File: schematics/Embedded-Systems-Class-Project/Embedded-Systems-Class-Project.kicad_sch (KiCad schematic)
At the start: 20 parts

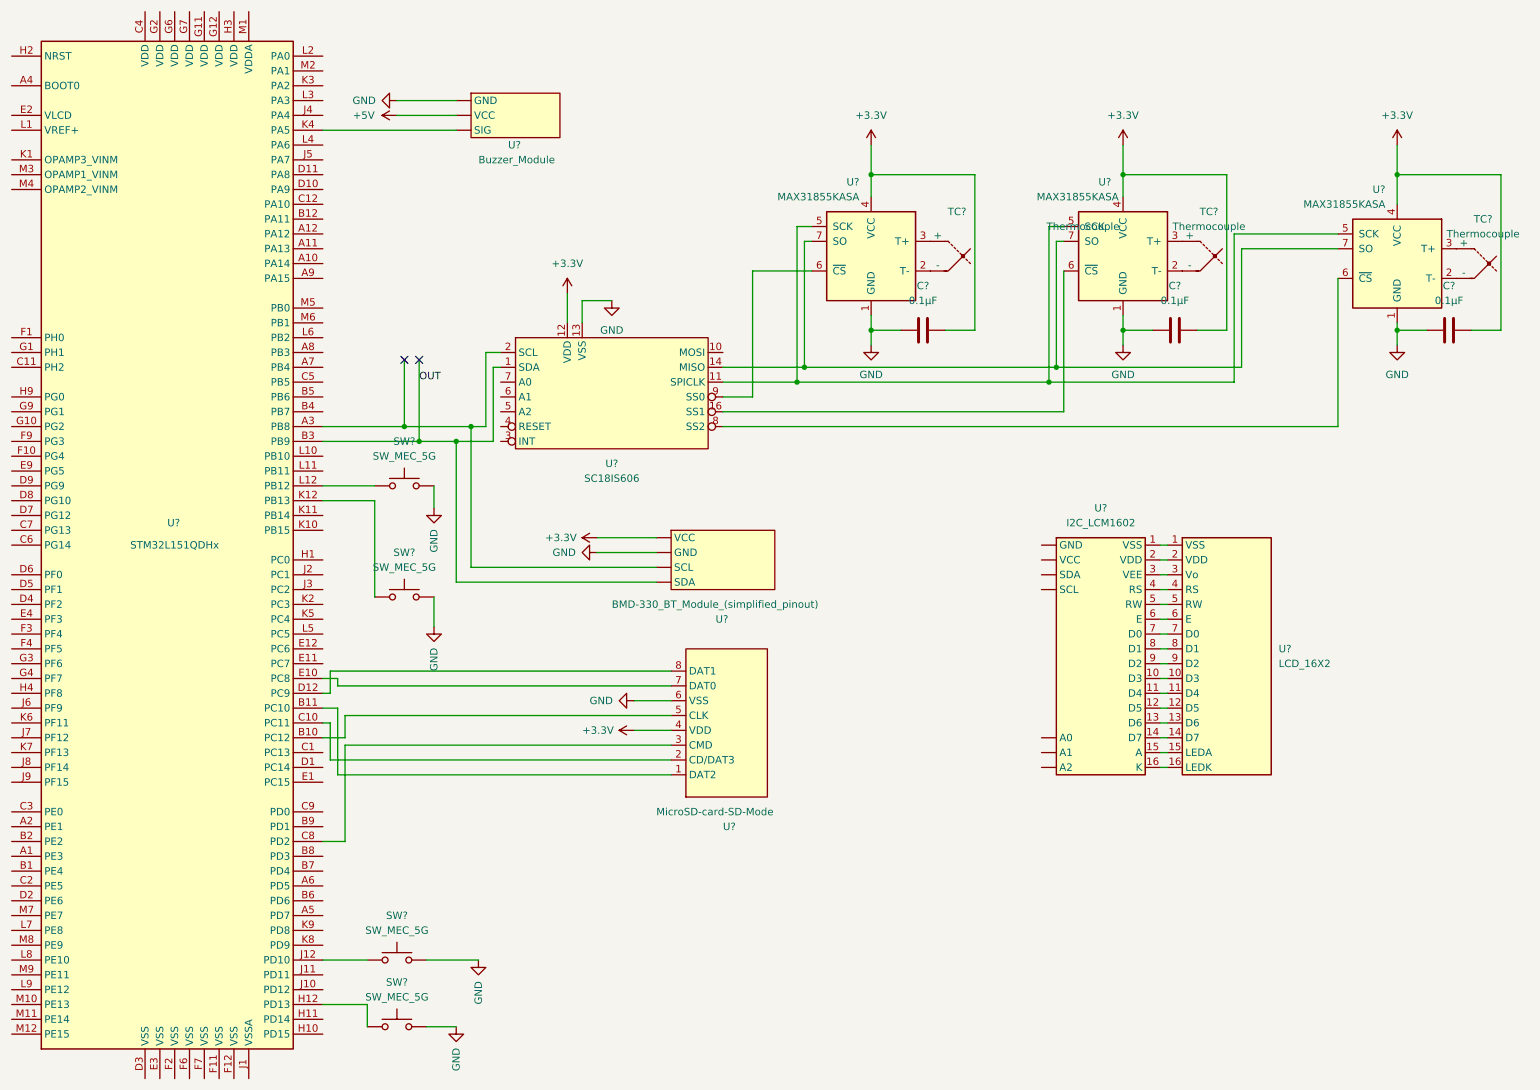
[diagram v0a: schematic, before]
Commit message: Update Embedded-Systems-Class-Project.kicad_sch
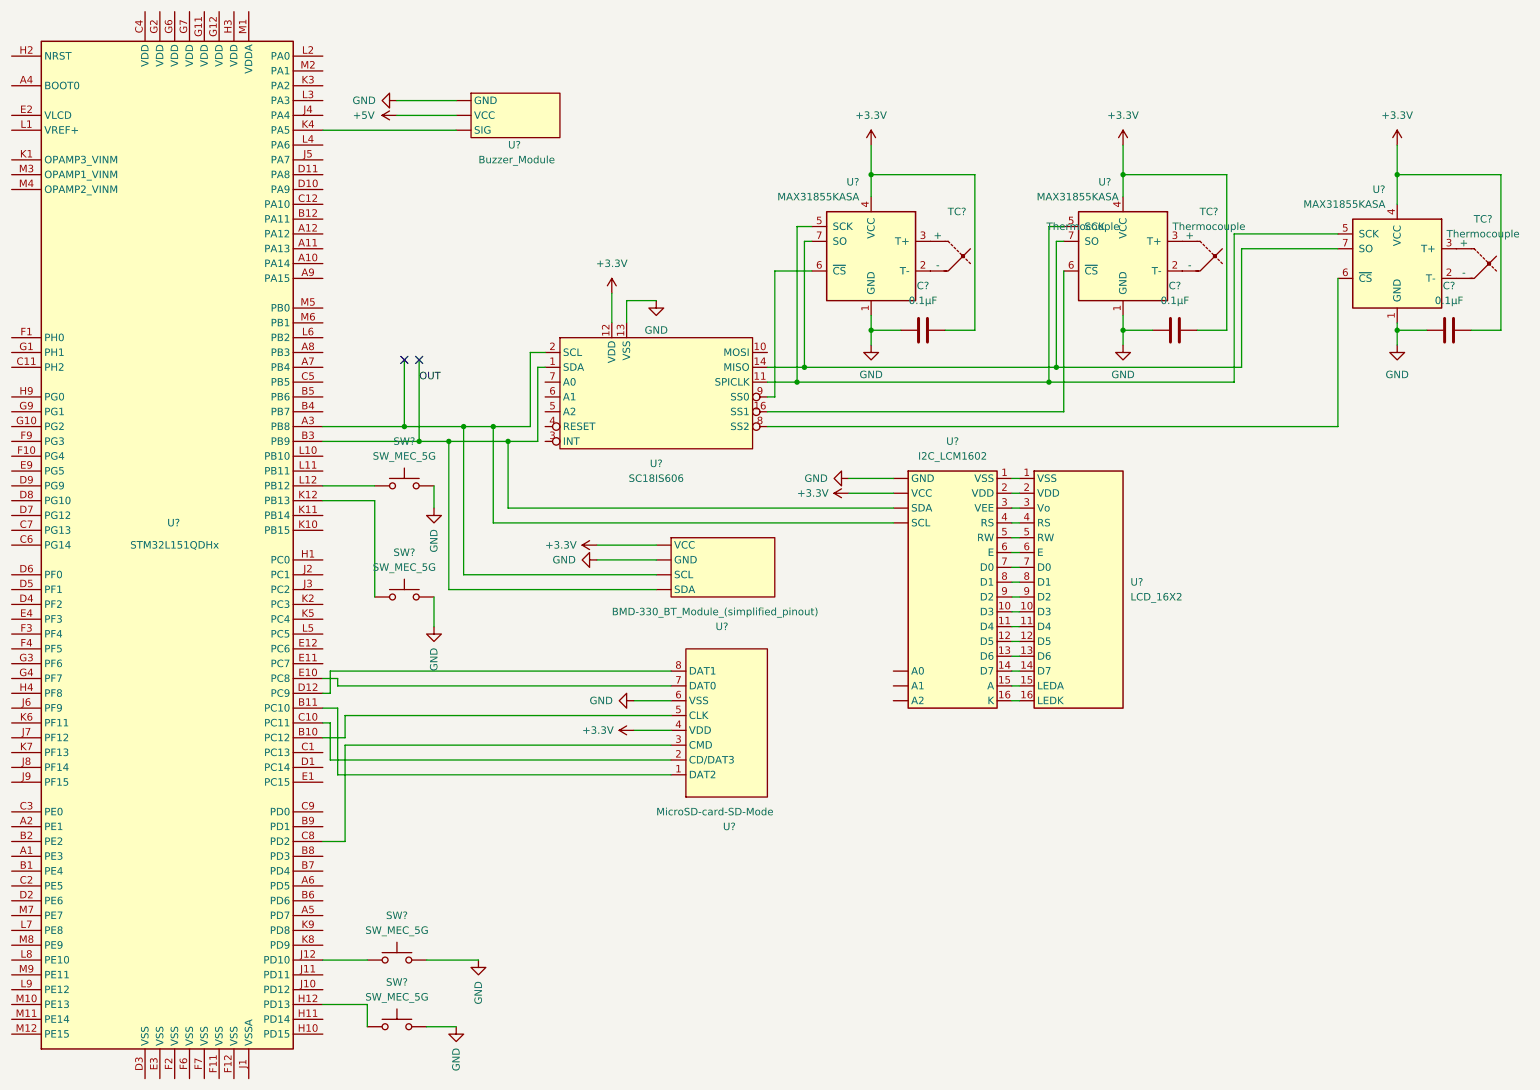
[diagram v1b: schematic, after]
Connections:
- net +3.3V: now also U?. (VCC)
- net GND: now also U?. (VCC)
- net OUT: now also U?. (VCC)
- net at U?. (VCC), U?.2 (SCL), U?.A3 (PB8): now also U?. (VCC)
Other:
- moved on the sheet: U?
